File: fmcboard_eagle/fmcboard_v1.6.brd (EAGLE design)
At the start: 147 x 74 mm, 281 parts, among them IC1 OPA699ID, IC10 LM358, IC11 7805DT, IC12 SN74AUC2G66DCTR, IC13 SN74AUC2G66DCTR, IC14 SN74AUC2G66DCTR, IC15 SN74AUC2G66DCTR, IC16 DAC7578SPWR, IC17 SN74AUC2G66DCTR, IC18 SN74AUC2G66DCTR, IC19 SN74AUC2G66DCTR, IC2 DAC7578SPWR, IC20 SN74AUC2G66DCTR, IC21 74AUP2GU04GW, IC22 74AUP2GU04GW, IC23 74AUP2GU04GW, IC24 74AUP2GU04GW, IC25 MC7905ACD2TR4G, IC26 AMS1117-1.8, IC27 LM358, IC28 SN74AUC2G66DCTR, IC29 LM337KVURG3, IC3 LTC6229IMS8E#TRPBF, IC30 SN74AUC2G66DCTR, IC31 SN74AUC2G66DCTR, IC32 SN74AUC2G66DCTR, IC33 LTC6229IMS8E#TRPBF, IC34 74AUP2GU04GW, IC35 74AUP2GU04GW, IC4 OPA695IDR, IC5 LTC6229IMS8E#TRPBF, IC6 OPA695IDR, IC7 OPA699ID, IC8 LM358, IC9 LM358, J1 8pin, J12 4p-2.54, J13 4p-2.54, J2 ASP-134604-01, J3 4p-2.54, J4 4p-2.54, J5 4p-2.54, J6 4p-2.54, J7 4p-2.54, J8 4p-2.54

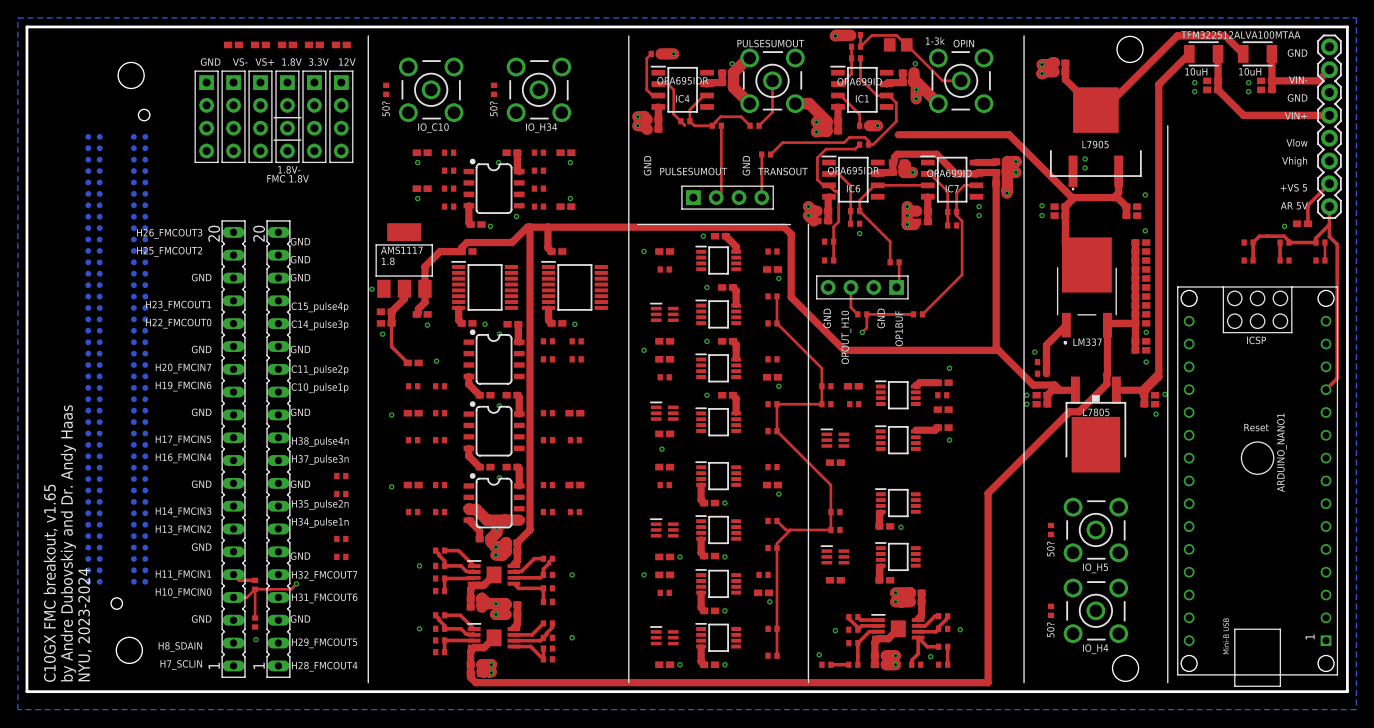
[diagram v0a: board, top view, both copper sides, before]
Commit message: routed
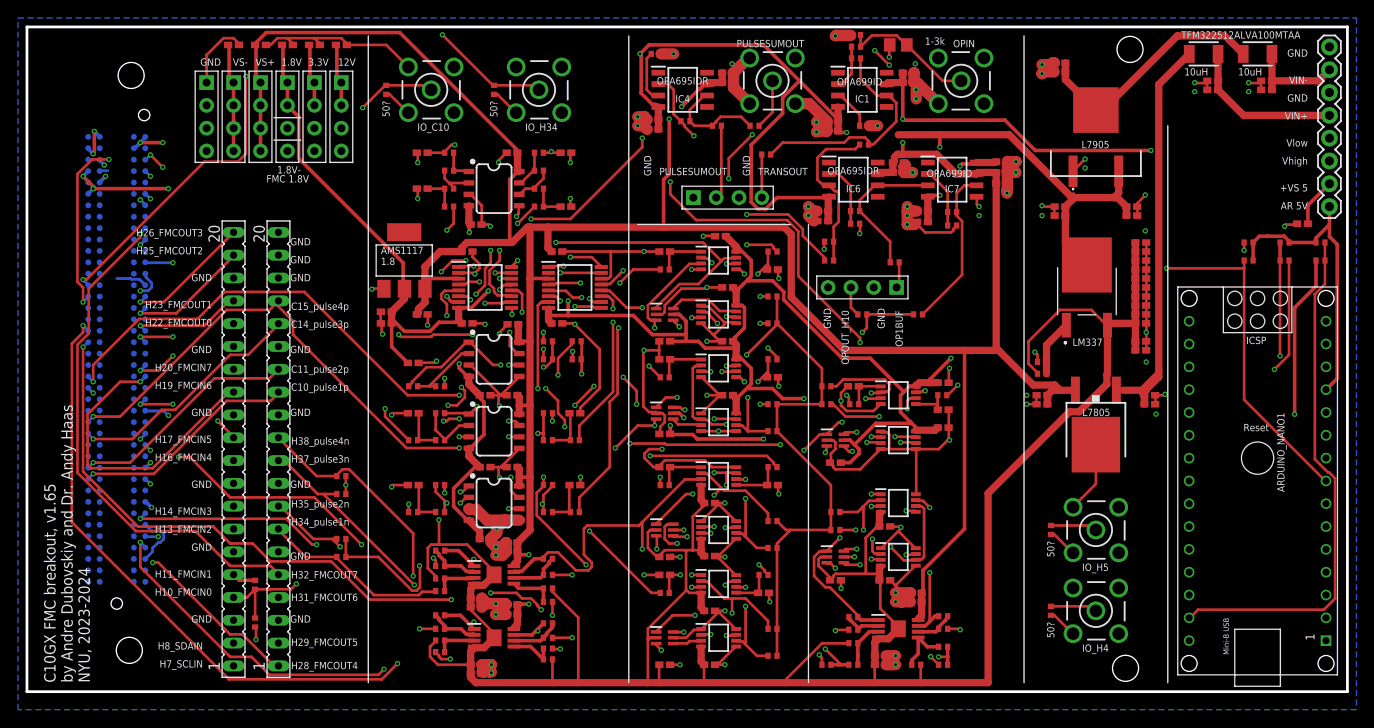
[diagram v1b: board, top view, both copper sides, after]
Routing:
- net GND: track 76.3 -> 448.3 mm, vias 102 -> 114
- net C27: track 0.00 -> 205.8 mm, vias 0 -> 2
- net 1V8: track 29.6 -> 229.8 mm, vias 0 -> 8
- net C26: track 0.00 -> 196.2 mm, vias 0 -> 4
- net 1V8-: track 159.3 -> 353.9 mm, vias 0 -> 1
- net VS-: track 62.2 -> 254.8 mm, vias 0 -> 6
- net SCLIN: track 0.00 -> 180.7 mm, vias 0 -> 3
- net VS+: track 197.1 -> 376.9 mm, vias 0 -> 7
- net SDAIN: track 0.00 -> 176.2 mm, vias 0 -> 2
- net AR_SCLIN2: track 0.00 -> 161.9 mm, vias 0 -> 3
- net H34: track 0.00 -> 134.1 mm, vias 0 -> 2
- net AR_SDAIN2: track 0.00 -> 133.9 mm, vias 0 -> 5
- net H5: track 0.00 -> 133.7 mm, vias 0 -> 1
- net C23: track 2.00 -> 132.5 mm, vias 0 -> 3
- net C19: track 0.00 -> 129.6 mm, vias 0 -> 4
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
